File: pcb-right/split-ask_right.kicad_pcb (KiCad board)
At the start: 2 copper layers, 165.5 x 98.7 mm, 59 parts, among them J1 MJ-4PP-9, SW1 SW_PUSH, SW10 SW_PUSH, SW11 SW_PUSH, SW12 SW_PUSH, SW13 SW_PUSH, SW14 SW_PUSH, SW15 SW_PUSH, SW16 SW_PUSH, SW17 SW_PUSH, SW18 SW_PUSH, SW19 SW_PUSH, SW2 SW_PUSH, SW20 SW_PUSH, SW21 SW_PUSH, SW22 SW_PUSH, SW23 SW_PUSH, SW24 SW_PUSH, SW25 SW_PUSH, SW26 SW_PUSH, SW27 SW_PUSH, SW28 SW_PUSH, SW3 SW_PUSH, SW4 SW_PUSH, SW5 SW_PUSH, SW6 SW_PUSH, SW7 SW_PUSH, SW8 SW_PUSH, SW9 SW_PUSH, U1 ProMicro

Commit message: update
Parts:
- added D29: D, kbd:D3_TH_SMD, F.Cu at (204.8, 109.5)
- added D30: D, kbd:D3_TH_SMD, F.Cu at (223.8, 109.5)
- added D31: D, kbd:D3_TH_SMD, F.Cu at (242.9, 109.5)
- added D32: D, kbd:D3_TH_SMD, F.Cu at (261.9, 109.5)
- added D33: D, kbd:D3_TH_SMD, F.Cu at (279.8, 109.5)
- added D34: D, kbd:D3_TH_SMD, F.Cu at (282.2, 109.5)
- added SW29: SW_PUSH, Alps_Only:ALPS-1U, F.Cu at (195.3, 109.5)
- added SW30: SW_PUSH, Alps_Only:ALPS-1U, F.Cu at (214.3, 109.5)
- added SW31: SW_PUSH, Alps_Only:ALPS-1U, F.Cu at (233.4, 109.5)
- added SW32: SW_PUSH, Alps_Only:ALPS-1U, F.Cu at (252.4, 109.5)
- added SW33: SW_PUSH, Alps_Only:ALPS-1U, F.Cu at (271.5, 109.5)
- added SW34: SW_PUSH, Alps_Only:ALPS-1U, F.Cu at (290.5, 109.5)
- SW13, SW27: footprint Alps_Only:ALPS-1.75U -> Alps_Only:ALPS-1U
- SW19: footprint Alps_Only:ALPS-2.25U -> Alps_Only:ALPS-1U
- SW28: footprint Alps_Only:ALPS-1U -> Alps_Only:ALPS-2.25U
- SW7: footprint Alps_Only:ALPS-1.5U -> Alps_Only:ALPS-1U
- SW8: footprint Alps_Only:ALPS-1U -> Alps_Only:ALPS-1.5U
- moved U1 251.7 mm to (286.3, 90.5), turned to 90 degrees
- moved SW7 224.6 mm to (261.9, 33.3)
- moved SW8 224.6 mm to (285.8, 33.3)
- moved D8 223.5 mm to (295.3, 33.3)
- moved D7 202.1 mm to (271.5, 33.3)
- moved SW13 193.8 mm to (233.4, 52.4)
- moved D14 186.7 mm to (261.9, 52.4)
- moved SW14 186.7 mm to (252.4, 52.4)
- moved D13 186.7 mm to (242.9, 52.4)
- moved SW15 186.7 mm to (271.5, 52.4)
- moved SW16 186.0 mm to (290.5, 62.5), turned to 90 degrees
- moved D15 185.5 mm to (279.8, 52.4)
- moved D26 177.2 mm to (238.1, 90.5)
- moved SW25 177.2 mm to (209.6, 90.5)
- moved D25 177.2 mm to (219.1, 90.5)
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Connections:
- D13 pad 1: row2 -> row1
- D14 pad 1: row2 -> row1
- D15 pad 1: row2 -> row1
- D16 pad 1: row2 -> row1
- D19 pad 1: row3 -> row2
- D20 pad 1: row3 -> row2
- D21 pad 1: row3 -> row2
- D22 pad 1: row3 -> row2
- D25 pad 1: row4 -> row3
- D26 pad 1: row4 -> row3
- D27 pad 1: row4 -> row3
- D28 pad 1: row4 -> row3
- D7 pad 1: row1 -> row0
- D8 pad 1: row1 -> row0
- SW10 pad 1: col3 -> col1
- SW11 pad 1: col4 -> col2
- SW12 pad 1: col5 -> col3
- SW13 pad 1: col0 -> col4
- SW14 pad 1: col1 -> col5
- SW15 pad 1: col2 -> col6
- SW16 pad 1: col3 -> col7
- SW17 pad 1: col4 -> col0
- SW18 pad 1: col5 -> col1
- SW19 pad 1: col0 -> col2
- SW20 pad 1: col1 -> col3
- SW21 pad 1: col2 -> col4
- SW22 pad 1: col3 -> col5
- SW23 pad 1: col4 -> col0
- SW24 pad 1: col5 -> col1
- SW25 pad 1: col0 -> col2
- SW26 pad 1: col1 -> col3
- SW27 pad 1: col2 -> col4
- SW28 pad 1: col3 -> col5
- SW7 pad 1: col0 -> col6
- SW8 pad 1: col1 -> col7
- SW9 pad 1: col2 -> col0
- U1 pad 13: Net-(U1-Pad13) -> col7
- U1 pad 14: Net-(U1-Pad14) -> col6
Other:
- board size 165.5 x 98.7 mm -> 165.4 x 98.7 mm

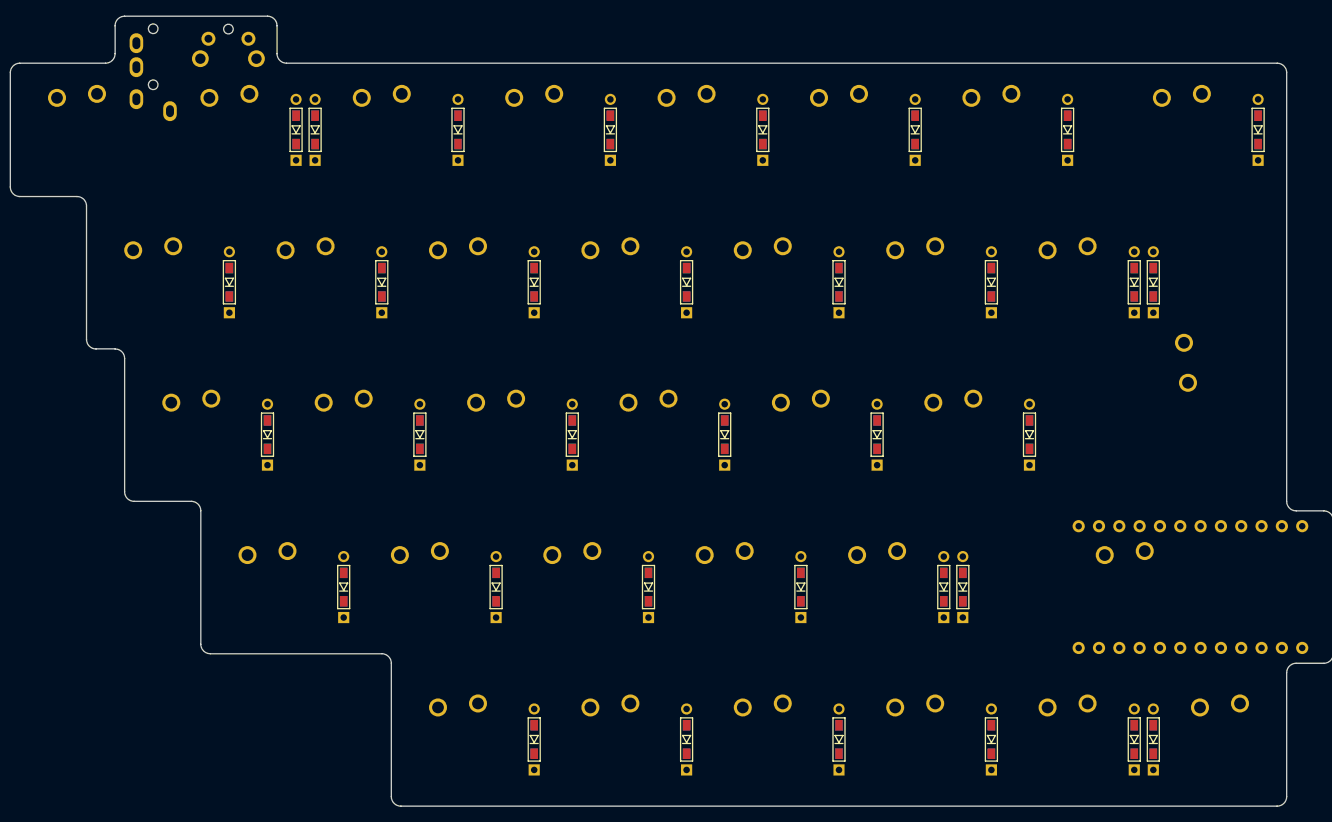
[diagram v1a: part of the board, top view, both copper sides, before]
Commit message: routing
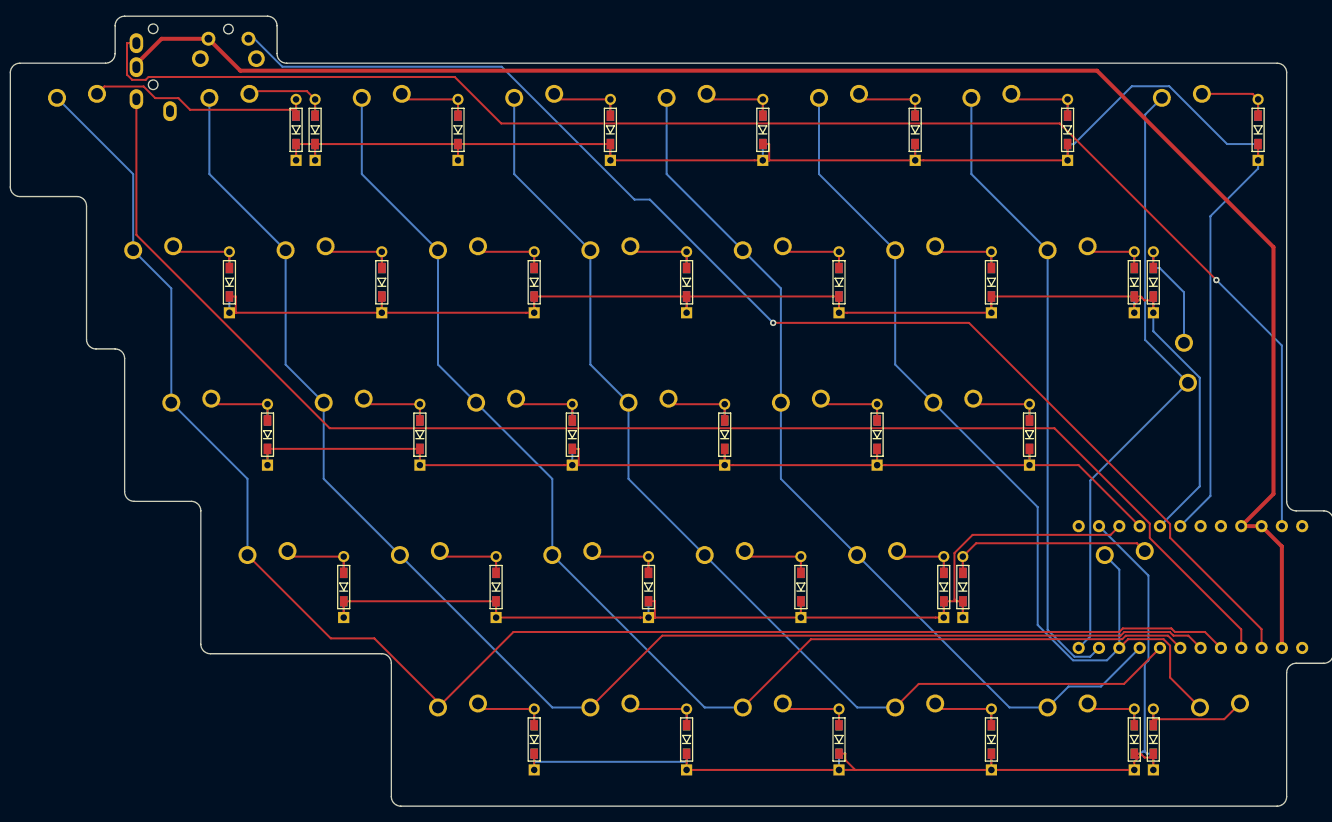
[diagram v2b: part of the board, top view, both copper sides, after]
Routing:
- net GND: track 0.00 -> 210.0 mm
- net row0: track 0.00 -> 209.7 mm
- net col0: track 0.00 -> 201.9 mm
- net data: track 0.00 -> 186.4 mm, vias 0 -> 1
- net row1: track 0.00 -> 180.5 mm
- net col1: track 0.00 -> 179.7 mm
- net VCC: track 0.00 -> 178.9 mm
- net reset: track 0.00 -> 160.6 mm, vias 0 -> 1
- net col2: track 0.00 -> 157.8 mm
- net row2: track 0.00 -> 137.6 mm
- net row4: track 0.00 -> 135.1 mm
- net col3: track 0.00 -> 134.9 mm
- net row3: track 0.00 -> 130.7 mm
- net col5: track 0.00 -> 118.7 mm
- net col4: track 0.00 -> 113.3 mm
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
